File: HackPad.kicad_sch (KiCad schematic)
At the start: 34 parts, among them J1 USB_C_Receptacle_USB2.0_16P, SW1 SW_Push, SW10 SW_Push, SW11 SW_Push, SW12 SW_Push, SW13 SW_Push, SW14 SW_Push, SW15 RotaryEncoder_Switch_MP, SW2 SW_Push, SW3 SW_Push, SW4 SW_Push, SW5 SW_Push, SW6 SW_Push, SW7 SW_Push, SW8 SW_Push, SW9 SW_Push, U1 ESP32-S3-WROOM-1U-N16R8, U2 COM-09032

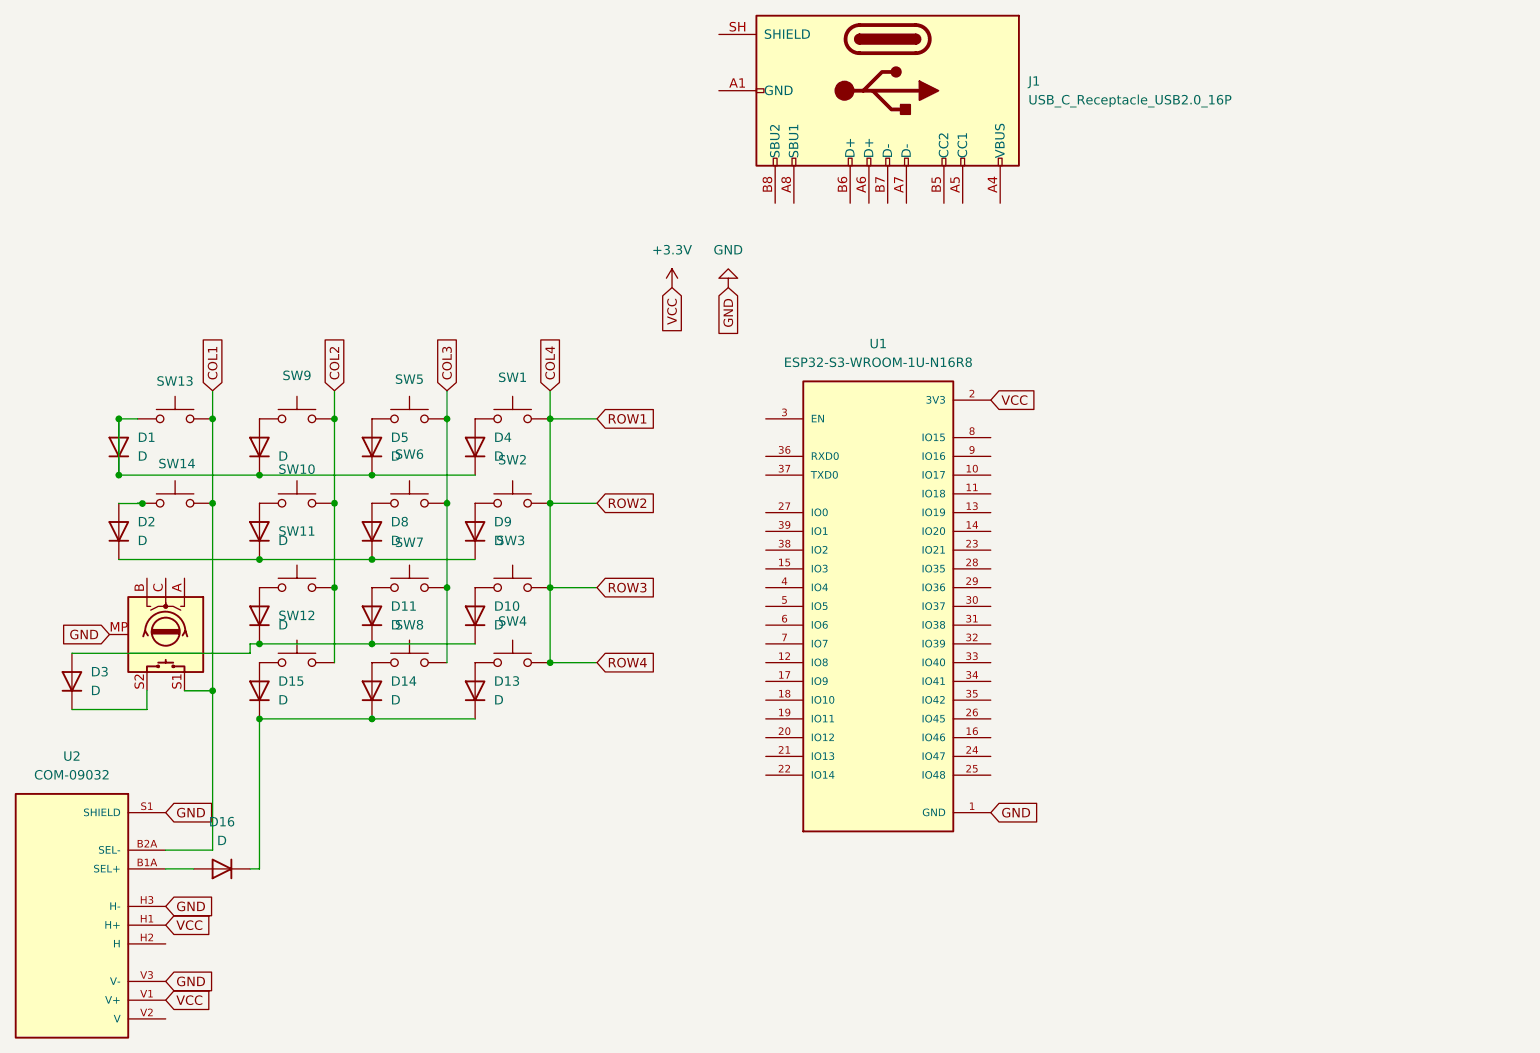
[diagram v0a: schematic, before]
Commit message: Finished the whole schematic. Started the PCB design.
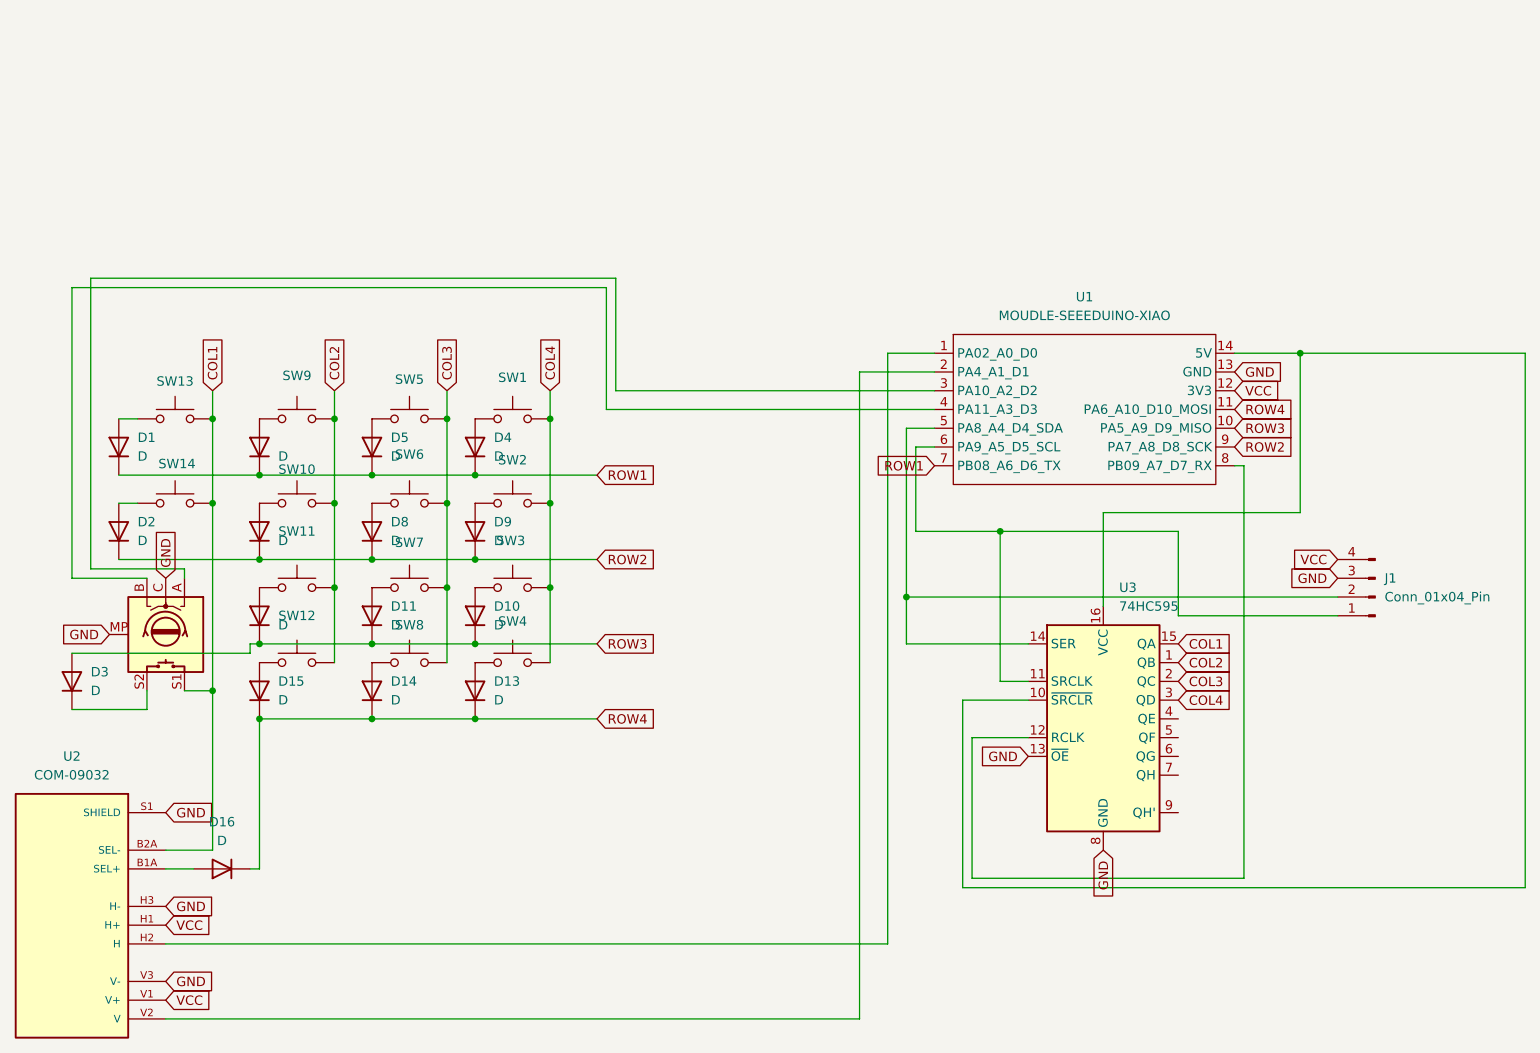
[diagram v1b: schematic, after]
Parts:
- removed J1: USB_C_Receptacle_USB2.0_16P, symbol Connector:USB_C_Receptacle_USB2.0_16P
- removed U1: ESP32-S3-WROOM-1U-N16R8, ESP32-S3-WROOM-1U-N16R8:XCVR_ESP32-S3-WROOM-1U-N16R8, symbol ESP32-S3-WROOM-1U-N16R8:ESP32-S3-WROOM-1U-N16R8
- added J1: Conn_01x04_Pin, Connector_PinHeader_2.54mm:PinHeader_1x04_P2.54mm_Vertical, symbol Connector:Conn_01x04_Pin
- added U1: MOUDLE-SEEEDUINO-XIAO, RF_Module:MCU_Seeed_ESP32C3, symbol XIAO_RP2040:MOUDLE-SEEEDUINO-XIAO
- added U3: 74HC595, Package_DIP:DIP-16_W7.62mm, symbol 74xx:74HC595
- D1, D10, D11, D12, D13, D14, D15, D16, D2, D3, D4, D5, D6, D7, D8, D9: footprint (none) -> Diode_THT:D_DO-35_SOD27_P7.62mm_Horizontal
- SW1, SW10, SW12, SW13, SW14, SW2, SW3, SW4, SW5, SW6, SW7, SW8, SW9: footprint (none) -> Button_Switch_Keyboard:SW_Cherry_MX_1.00u_PCB
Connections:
- net COL1: now also U3.15 (QA)
- net COL2: now also U3.1 (QB)
- net COL3: now also U3.2 (QC)
- net COL4: now also U3.3 (QD)
- net GND: now also SW15.C, J1.3 (Pin_3), U1.13 (GND), U3.13 (~{OE}), U3.8 (GND)
- net at U2.H2 (H): now also U1.1 (PA02_A0_D0)
- net at U2.V2 (V): now also U1.2 (PA4_A1_D1)
- net ROW2: now reaches D2.1 (K), D7.1 (K), D8.1 (K), D9.1 (K)
- net ROW2: now also U1.9 (PA7_A8_D8_SCK)
- net at D2.2 (A): now also SW14.1
- net ROW4: now reaches D13.1 (K), D14.1 (K), D15.1 (K), D16.1 (K)
- net ROW4: now also U1.11 (PA6_A10_D10_MOSI)
- net ROW3: now reaches D10.1 (K), D11.1 (K), D12.1 (K), D3.2 (A)
- net ROW3: now also U1.10 (PA5_A9_D9_MISO)
- net ROW1: now reaches D1.1 (K), D4.1 (K), D5.1 (K), D6.1 (K)
- net ROW1: now also U1.7 (PB08_A6_D6_TX); no longer D1.2 (A), SW13.1
- net at SW15.A: now also U1.3 (PA10_A2_D2)
- net at SW15.B: now also U1.4 (PA11_A3_D3)
- net +3.3V renamed VCC
- net VCC: now also J1.4 (Pin_4), U1.12 (3V3)
- new net: D1.2 (A), SW13.1
- new net: U1.14 (5V), U3.10 (~{SRCLR}), U3.16 (VCC)
- new net: J1.2 (Pin_2), U1.5 (PA8_A4_D4_SDA), U3.14 (SER)
- new net: J1.1 (Pin_1), U1.6 (PA9_A5_D5_SCL), U3.11 (SRCLK)
- new net: U1.8 (PB09_A7_D7_RX), U3.12 (RCLK)
